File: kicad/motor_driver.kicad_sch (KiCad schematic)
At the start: 1 part

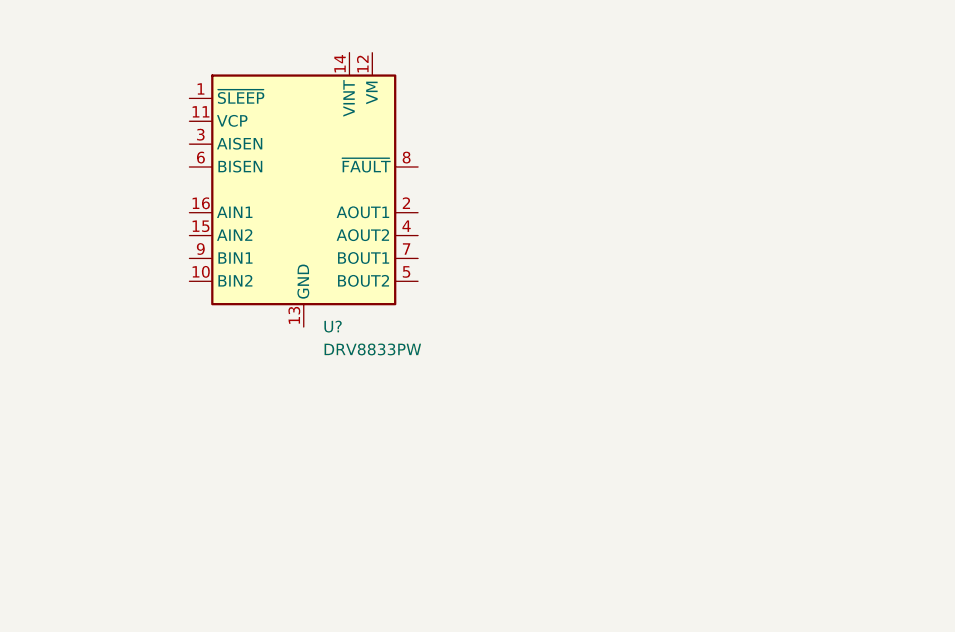
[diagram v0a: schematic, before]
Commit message: init
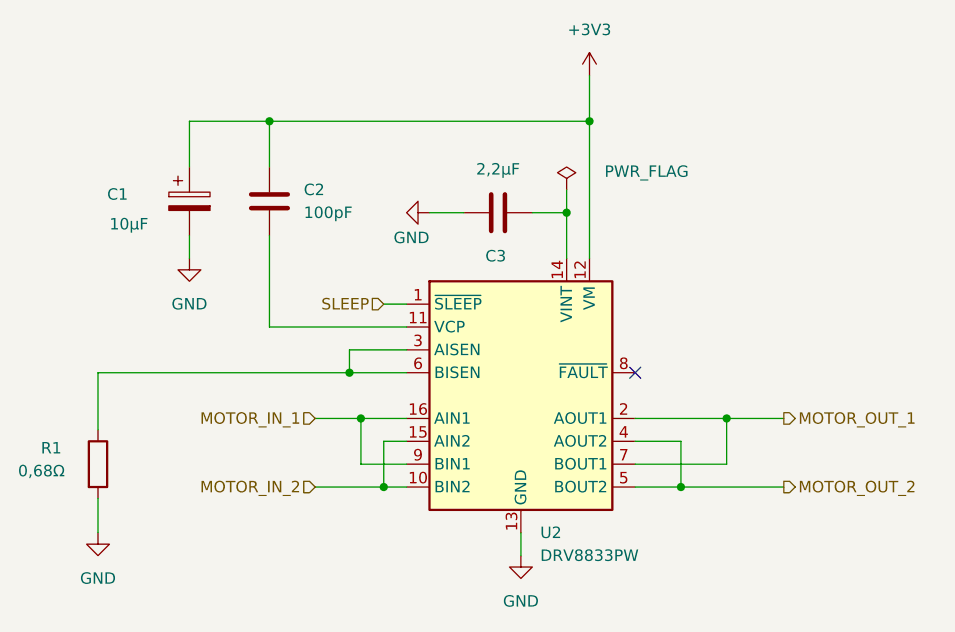
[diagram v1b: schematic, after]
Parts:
- removed U?: DRV8833PW, Package_SO:TSSOP-16_4.4x5mm_P0.65mm, symbol Driver_Motor:DRV8833PW
- added C1: 10µF, Capacitor_THT:CP_Radial_D5.0mm_P2.00mm, symbol Device:C_Polarized
- added C2: 100pF, Capacitor_SMD:C_1206_3216Metric, symbol Device:C
- added C3: 2,2µF, Capacitor_SMD:C_1206_3216Metric, symbol Device:C
- added R1: 0,68Ω, Resistor_SMD:R_1206_3216Metric, symbol Device:R
- added U2: DRV8833PW, Package_SO:TSSOP-16_4.4x5mm_P0.65mm, symbol Driver_Motor:DRV8833PW
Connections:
- new net: R1.1, U2.3 (AISEN), U2.6 (BISEN)
- new net: C3.2, U2.14 (VINT)
- new net: C2.2, U2.11 (VCP)
- new net +3V3: C1.1, C2.1, U2.12 (VM)
- new net GND: C1.2, C3.1, R1.2, U2.13 (GND)
- new net MOTOR_IN_1: U2.16 (AIN1), U2.9 (BIN1)
- new net MOTOR_IN_2: U2.10 (BIN2), U2.15 (AIN2)
- new net MOTOR_OUT_1: U2.2 (AOUT1), U2.7 (BOUT1)
- new net MOTOR_OUT_2: U2.4 (AOUT2), U2.5 (BOUT2)
- new net SLEEP: U2.1 (~{SLEEP})
- no-connect marks 0 -> 1
